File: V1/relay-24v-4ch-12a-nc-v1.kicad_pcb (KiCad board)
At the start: 2 copper layers, 53 x 67.8 mm, 23 parts, among them J1 DG141V-2.54-6P, J2 DB142V-5.08-4P, J3 DB142V-5.08-4P, K1 Songle_SRD_1B, K2 Songle_SRD_1B, K3 Songle_SRD_1B, K4 Songle_SRD_1B

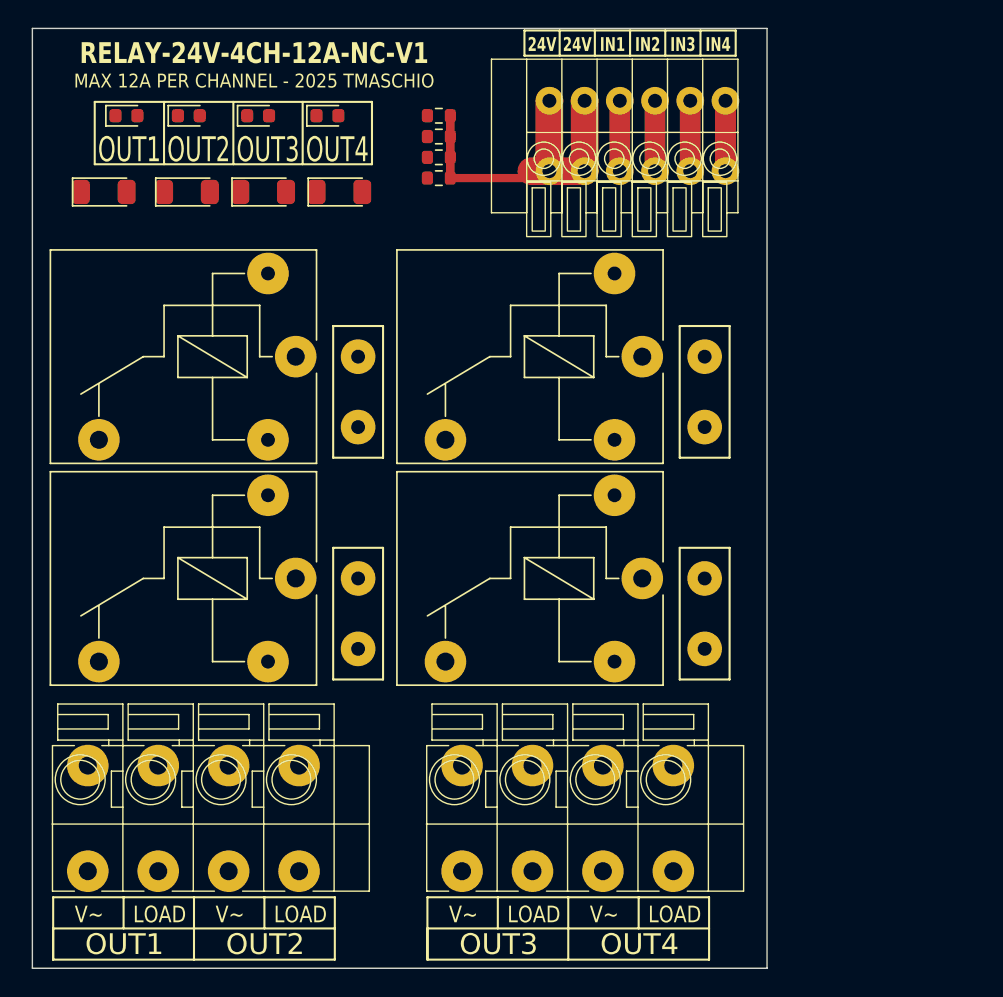
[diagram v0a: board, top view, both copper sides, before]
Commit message: Creating layout
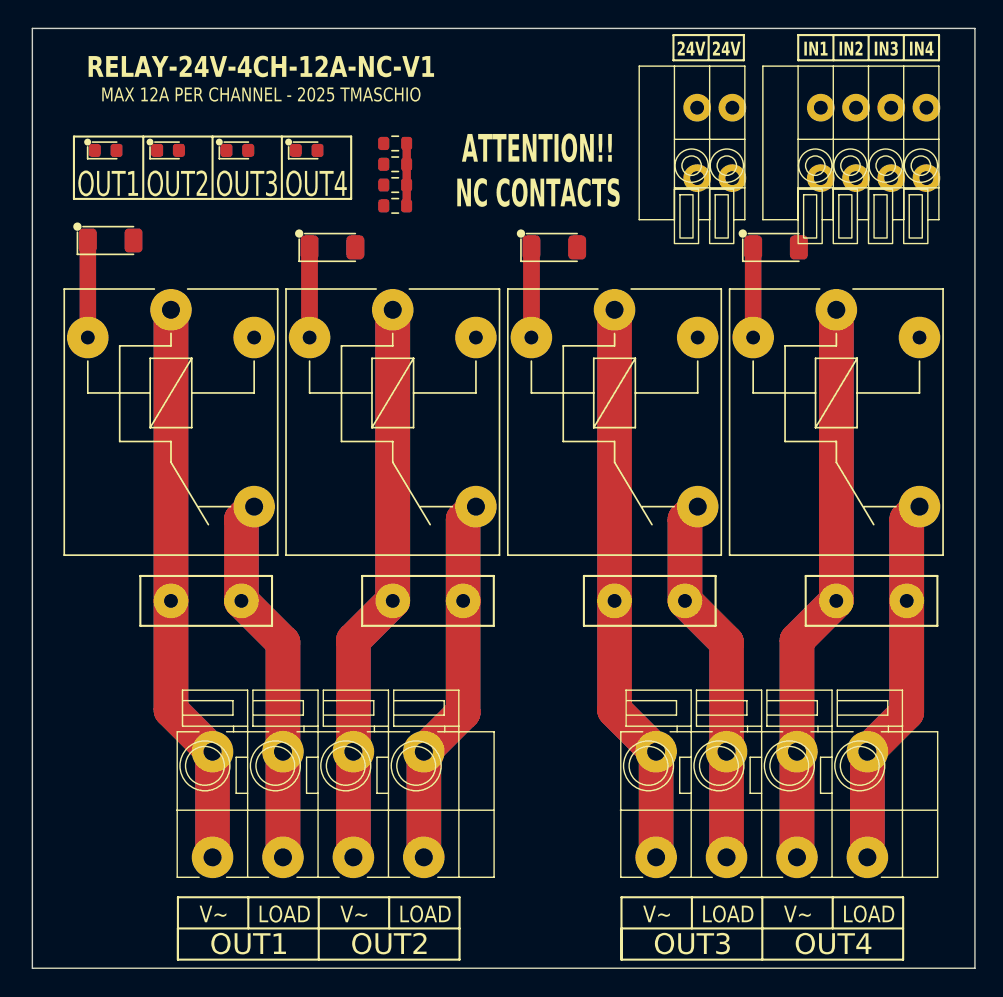
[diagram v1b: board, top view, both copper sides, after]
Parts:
- added J2: DB141V-2.54-4P, Tales:TerminalBlock_Dibo_DB141V-2.54-4P_1x04_P2.54mm_Vertical, F.Cu at (189.5, 67.9)
- J1: value DG141V-2.54-6P -> DB141V-2.54-2P; footprint Tales:TerminalBlock_Dibo_DB141V-2.54-6P_1x06_P2.54mm_Vertical -> Tales:TerminalBlock_Dibo_DB141V-2.54-2P_1x02_P2.54mm_Vertical
- moved D8 31.8 mm to (178.7, 78.0)
- moved K4 23.9 mm to (183.0, 82.5), turned to -90 degrees
- moved RV1 22.2 mm to (135.0, 103.5), turned to 0 degrees
- moved D6 21.4 mm to (162.7, 78.0)
- moved K2 20.6 mm to (151.0, 82.5), turned to -90 degrees
- moved RV3 18.8 mm to (167.0, 103.5), turned to 0 degrees
- moved J4 14.0 mm to (170.0, 122.0)
- moved D4 11.2 mm to (146.7, 78.0)
- moved RV4 9.64 mm to (183.0, 103.5), turned to 0 degrees
- moved K1 9.61 mm to (135.0, 82.5), turned to -90 degrees
- moved J3 9.06 mm to (138.0, 122.0)
- moved K3 3.93 mm to (167.0, 82.5), turned to -90 degrees
- moved R1 3.73 mm to (151.2, 70.5)
- moved R2 3.73 mm to (151.2, 72.0)
- moved R3 3.73 mm to (151.2, 73.5)
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- renumbered J2 to J3, J3 to J4
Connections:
- J1 pad 1: Net-(D7-K) -> +24V
- J1 pad 2: Net-(D5-K) -> +24V
- J3 pad 2: Net-(J2-Pin_2) -> Net-(J3-Pin_2)
- J3 pad 4: Net-(J2-Pin_4) -> Net-(J3-Pin_4)
- J4 pad 2: Net-(J3-Pin_2) -> Net-(J4-Pin_2)
- J4 pad 4: Net-(J3-Pin_4) -> Net-(J4-Pin_4)
- RV1 pad 2: Net-(J2-Pin_2) -> Net-(J3-Pin_2)
- RV2 pad 2: Net-(J2-Pin_4) -> Net-(J3-Pin_4)
- RV3 pad 2: Net-(J3-Pin_2) -> Net-(J4-Pin_2)
- RV4 pad 2: Net-(J3-Pin_4) -> Net-(J4-Pin_4)
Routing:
- net Net-(J4-Pin_1): track 0.00 -> 81.5 mm
- net Net-(J3-Pin_1): track 0.00 -> 81.5 mm
- net Net-(J4-Pin_3): track 0.00 -> 81.4 mm
- net Net-(J3-Pin_3): track 0.00 -> 81.4 mm
- net Net-(J4-Pin_2): track 0.00 -> 53.8 mm
- net Net-(J3-Pin_2): track 0.00 -> 53.8 mm
- net Net-(J4-Pin_4): track 0.00 -> 53.7 mm
- net Net-(J3-Pin_4): track 0.00 -> 53.7 mm
- net +24V: track 24.3 -> 31.0 mm
- net Net-(D7-K): track 5.08 -> 0.00 mm
- net Net-(D5-K): track 5.08 -> 0.00 mm
- net Net-(D3-K): track 5.08 -> 0.00 mm
- net Net-(D1-K): track 5.08 -> 0.00 mm
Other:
- board size 53 x 67.8 mm -> 68 x 67.8 mm
- board text added: "ATTENTION!! NC CONTACTS"
- board text added: "SUPORTES PCI METALTEX SP7 1x pé macho 9 mm 1x pé fêmea 9 mm 1x espaçador 30 mm 1x espaçador 20 mm Comprimento total 68 mm Largura da placa 67,8 mm"
- board text removed: "SUPORTES PCI METALTEX SP7 1x pé macho 9 mm 1x pé fêmea 9 mm 1x espaçador 30 mm 1x espaçador 5 mm Comprimento total 53 mm Largura da placa 67,8 mm"
